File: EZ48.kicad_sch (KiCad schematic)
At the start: 13 parts, among them IC1 2732, IC2 2732, IC3 2732, U1 74LS139, U2 74LS06, U3 NE556, U4 6502, U5 74LS138

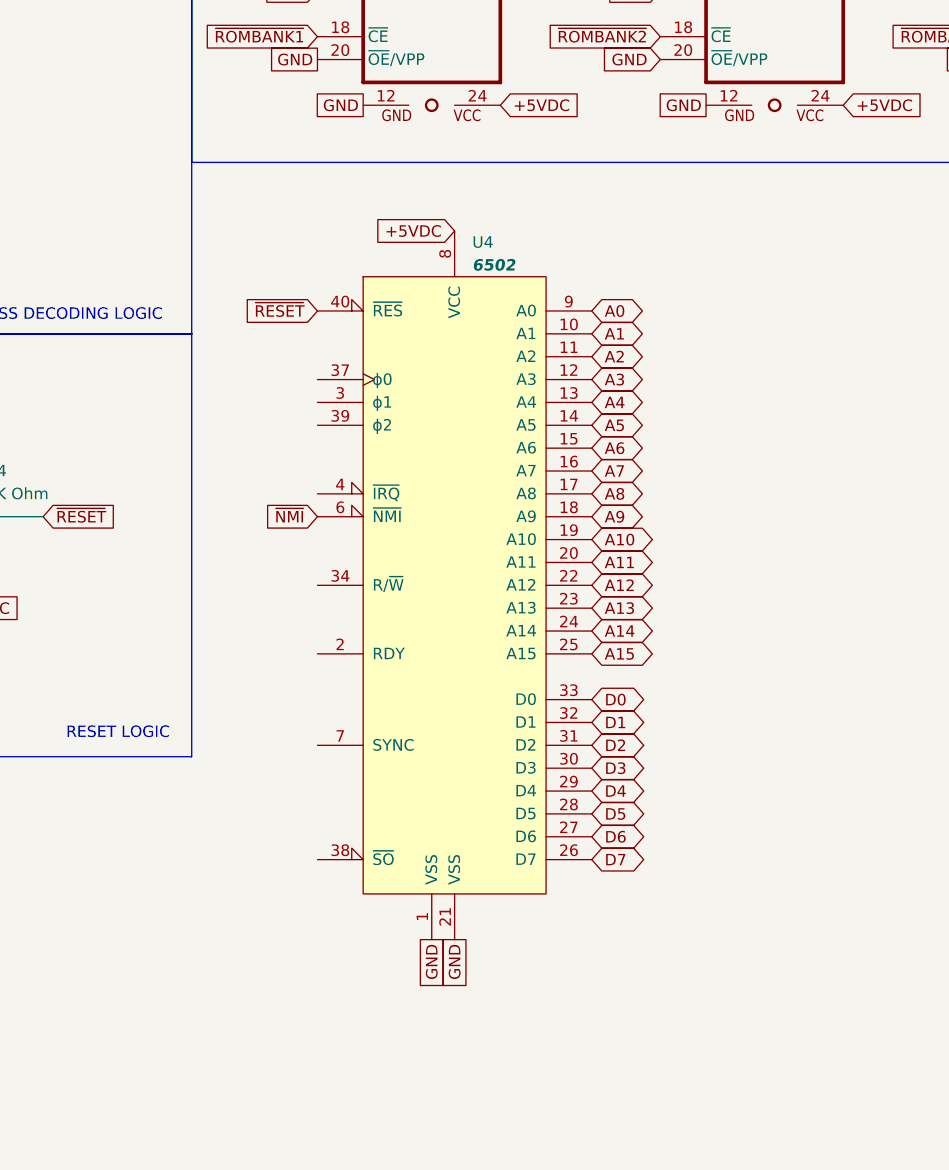
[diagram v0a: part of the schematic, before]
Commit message: Add files via upload
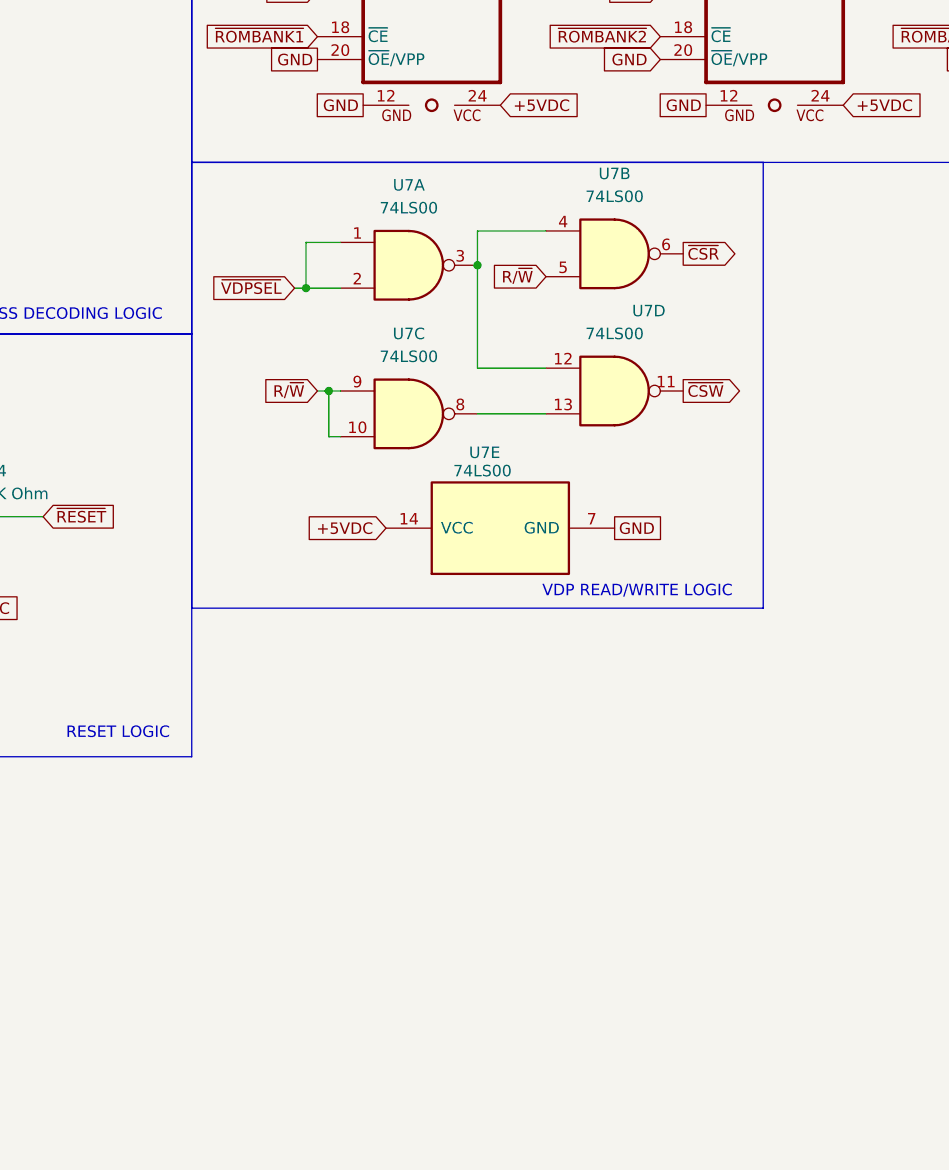
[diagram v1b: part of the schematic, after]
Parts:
- removed U4: 6502, Package_DIP:DIP-40_W15.24mm_LongPads, symbol 65xx:6502
- added U7: 74LS00, Package_DIP:DIP-14_W7.62mm_LongPads, symbol 74xx:74LS00
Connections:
- net +5VDC: now also U7.14 (VCC)
- net GND: now also U7.7 (GND)
- net ~{VDPSEL}: now also U7.1, U7.2
- new net: U7.12, U7.3, U7.4
- new net: U7.13, U7.8
- new net R/~{W}: U7.10, U7.5, U7.9
- new net ~{CSR}: U7.6
- new net ~{CSW}: U7.11
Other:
- note added: "VDP READ/WRITE LOGIC"

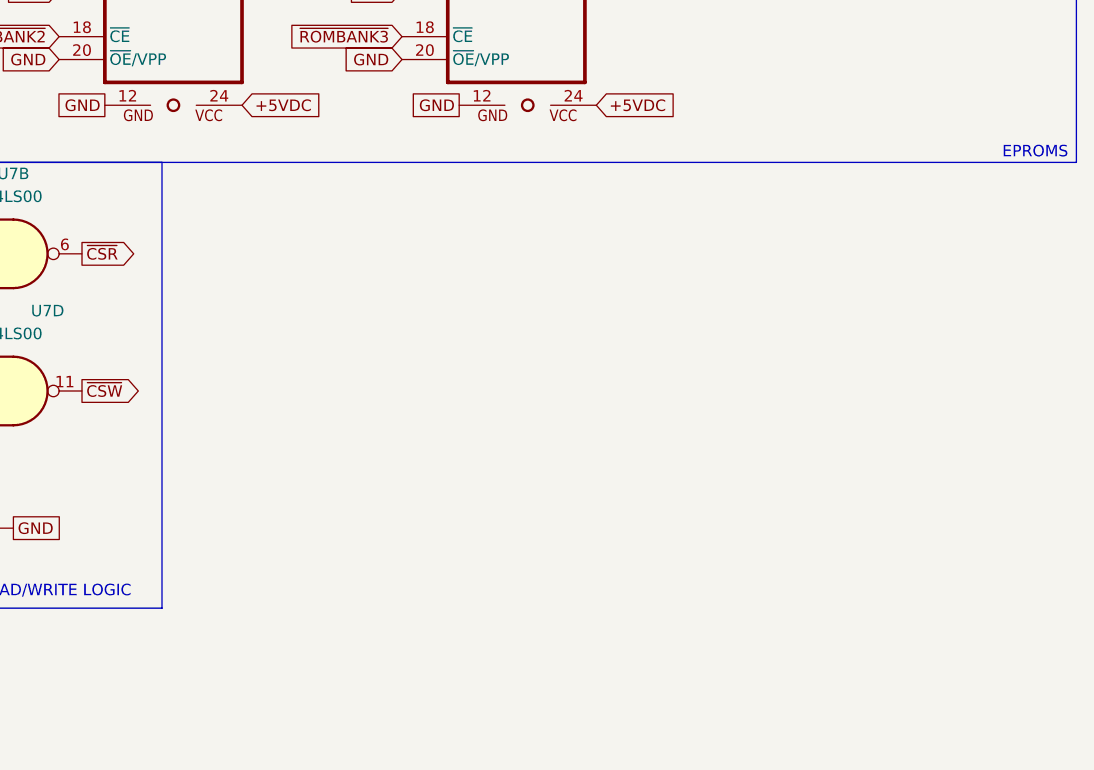
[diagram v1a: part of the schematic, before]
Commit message: Add files via upload
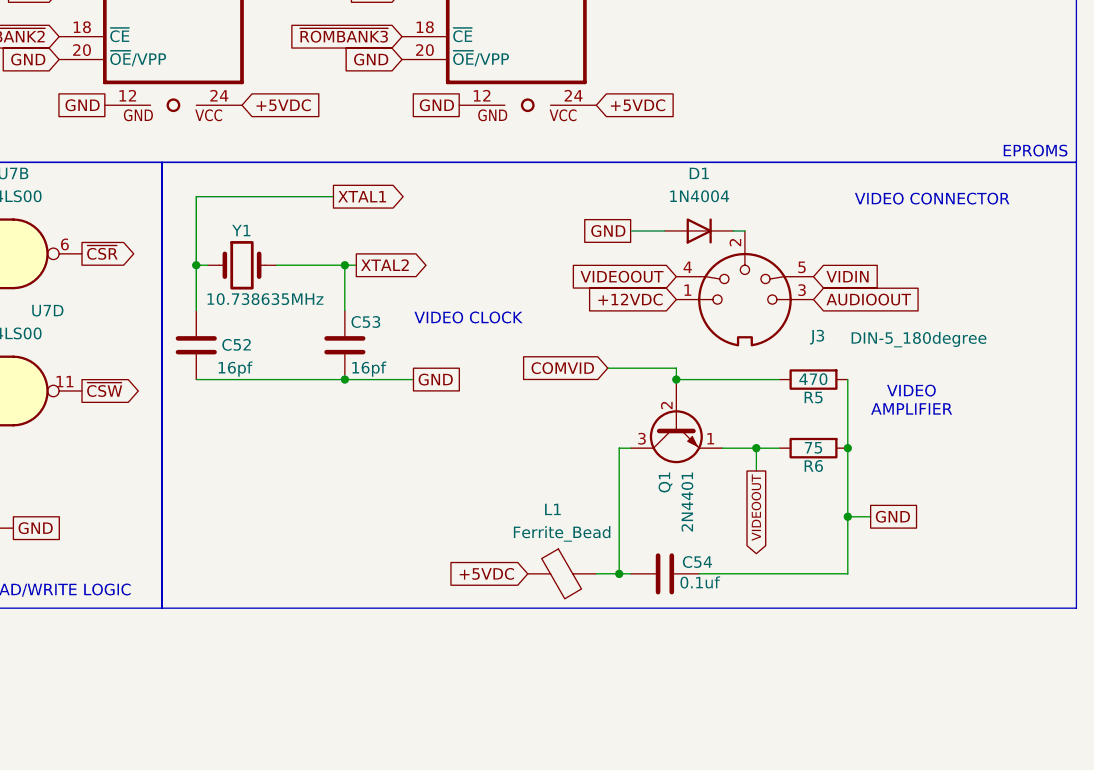
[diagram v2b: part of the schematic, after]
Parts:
- added C52, C53: 16pf, Capacitor_THT:C_Disc_D3.0mm_W1.6mm_P2.50mm, symbol Device:C
- added C54: 0.1uf, Capacitor_THT:C_Disc_D3.0mm_W1.6mm_P2.50mm, symbol Device:C
- added D1: 1N4004, Diode_THT:D_DO-41_SOD81_P10.16mm_Horizontal, symbol Diode:1N4004
- added J3: DIN-5_180degree, w_conn_av:din-5, symbol Connector:DIN-5_180degree
- added L1: Ferrite_Bead, Resistor_THT:R_Axial_DIN0207_L6.3mm_D2.5mm_P7.62mm_Horizontal, symbol Device:Ferrite_Bead
- added Q1: 2N4401, Package_TO_SOT_THT:TO-92, symbol Device:Q_NPN_EBC
- added R5: 470, Resistor_THT:R_Axial_DIN0207_L6.3mm_D2.5mm_P7.62mm_Horizontal, symbol Device:R
- added R6: 75, Resistor_THT:R_Axial_DIN0207_L6.3mm_D2.5mm_P7.62mm_Horizontal, symbol Device:R
- added Y1: 10.738635MHz, Crystal:Crystal_HC49-4H_Vertical, symbol Device:Crystal
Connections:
- net +5VDC: now also L1.1
- net GND: now also C52.2, C53.2, C54.2, D1.2 (A), R5.2, R6.2
- new net: C54.1, L1.2, Q1.3 (C)
- new net: D1.1 (K), J3.2
- new net +12VDC: J3.1
- new net AUDIOOUT: J3.3
- new net COMVID: Q1.2 (B), R5.1
- new net VIDEOOUT: J3.4, Q1.1 (E), R6.1
- new net VIDIN: J3.5
- new net XTAL1: C52.1, Y1.1
- new net XTAL2: C53.1, Y1.2
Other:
- note added: "VIDEO AMPLIFIER"
- note added: "VIDEO CLOCK"
- note added: "VIDEO CONNECTOR"

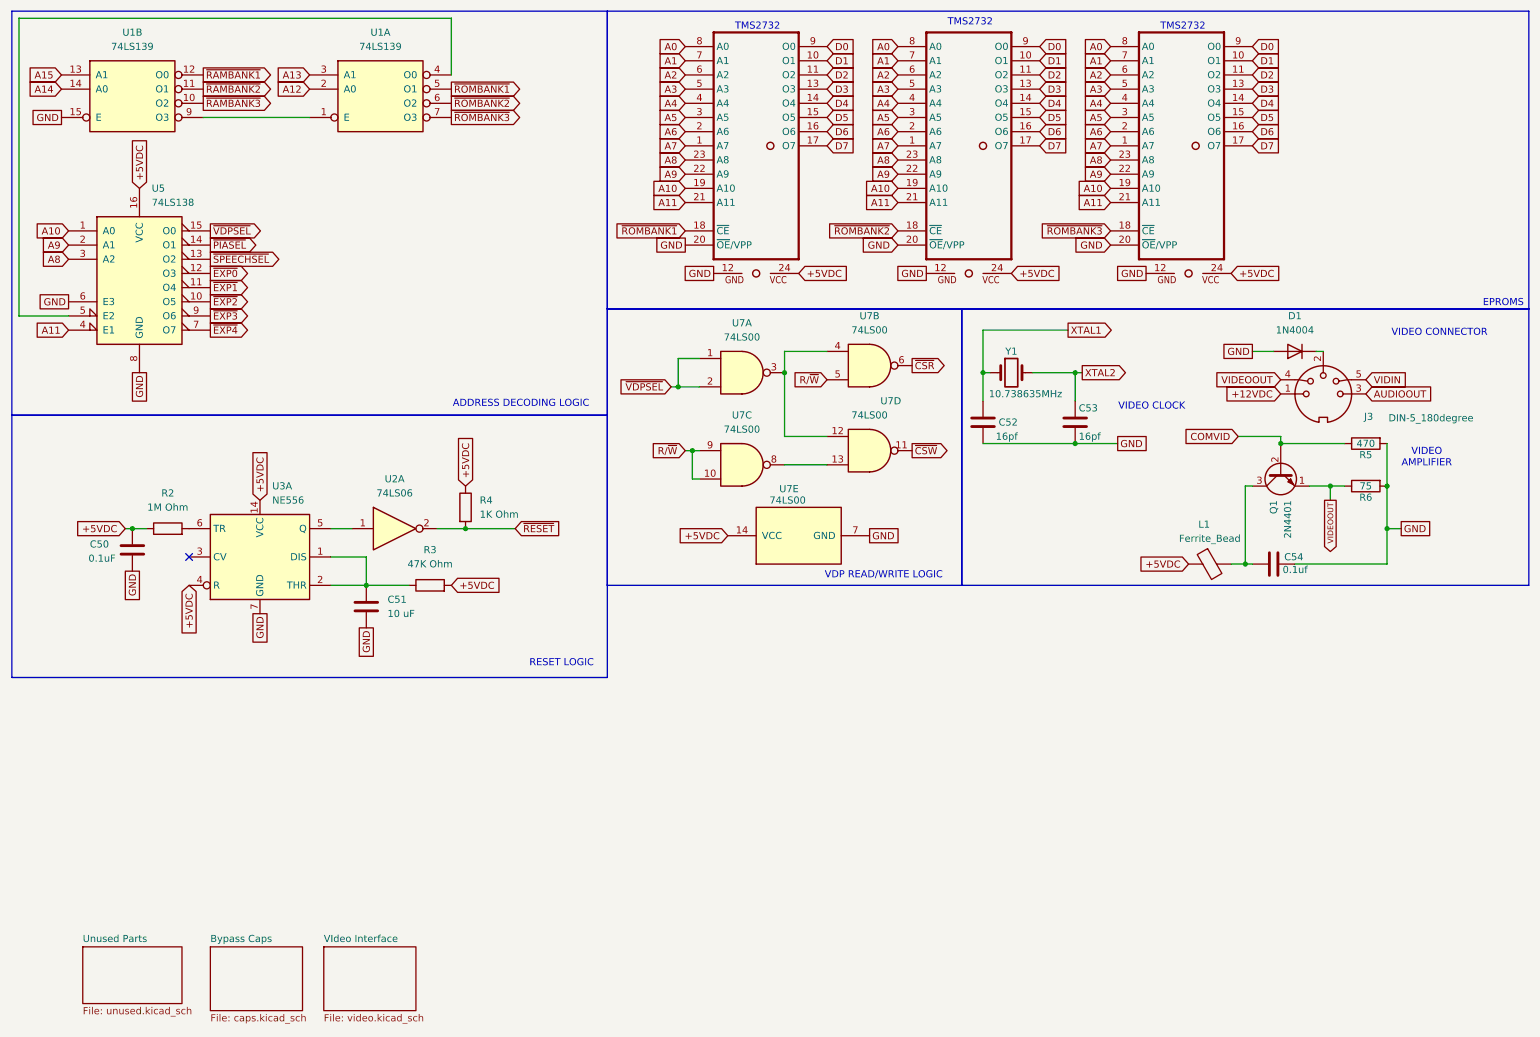
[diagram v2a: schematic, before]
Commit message: Add files via upload
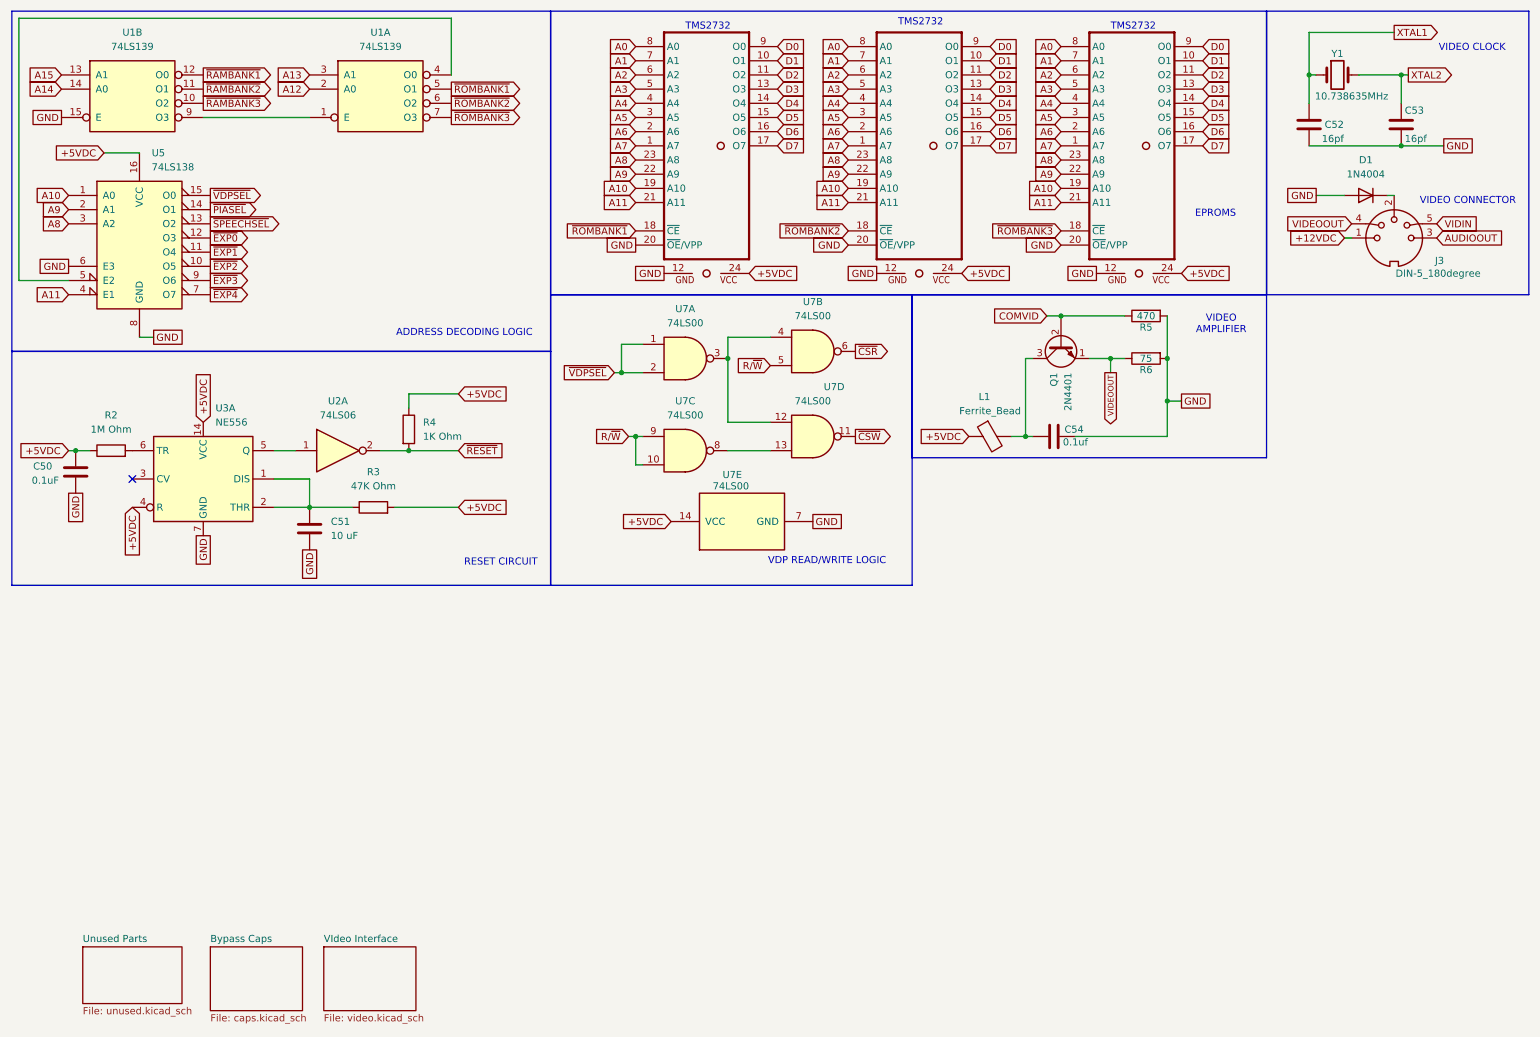
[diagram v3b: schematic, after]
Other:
- note added: "RESET CIRCUIT"
- note removed: "RESET LOGIC"
- moved on the sheet: C50, C51, C52, C53, C54, D1, J3, L1, Q1, R2, R3, R4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
